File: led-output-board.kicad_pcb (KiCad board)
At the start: 2 copper layers, 80.9 x 96.4 mm, 29 parts, among them J1 DBT50G-9.5-2P, J10 DB301V-3.5-3P-GN, J2 Conn_02x08_Odd_Even, J3 DB301V-3.5-3P-GN, J4 DB301V-3.5-3P-GN, J5 DB301V-3.5-3P-GN, J6 DB301V-3.5-3P-GN, J7 DB301V-3.5-3P-GN, J8 DB301V-3.5-3P-GN, J9 DB301V-3.5-3P-GN, U1 SN74LVC8T245PWR

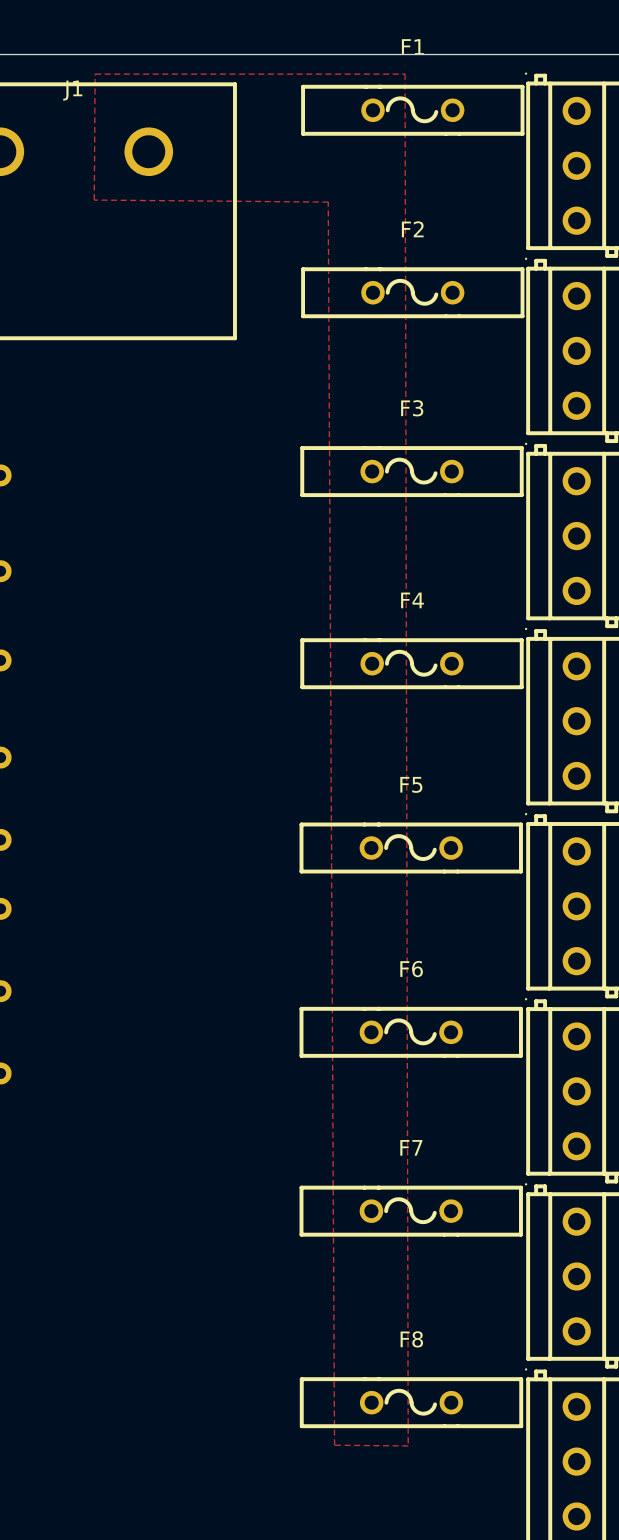
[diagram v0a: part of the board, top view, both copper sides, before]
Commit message: Widened and filled zone
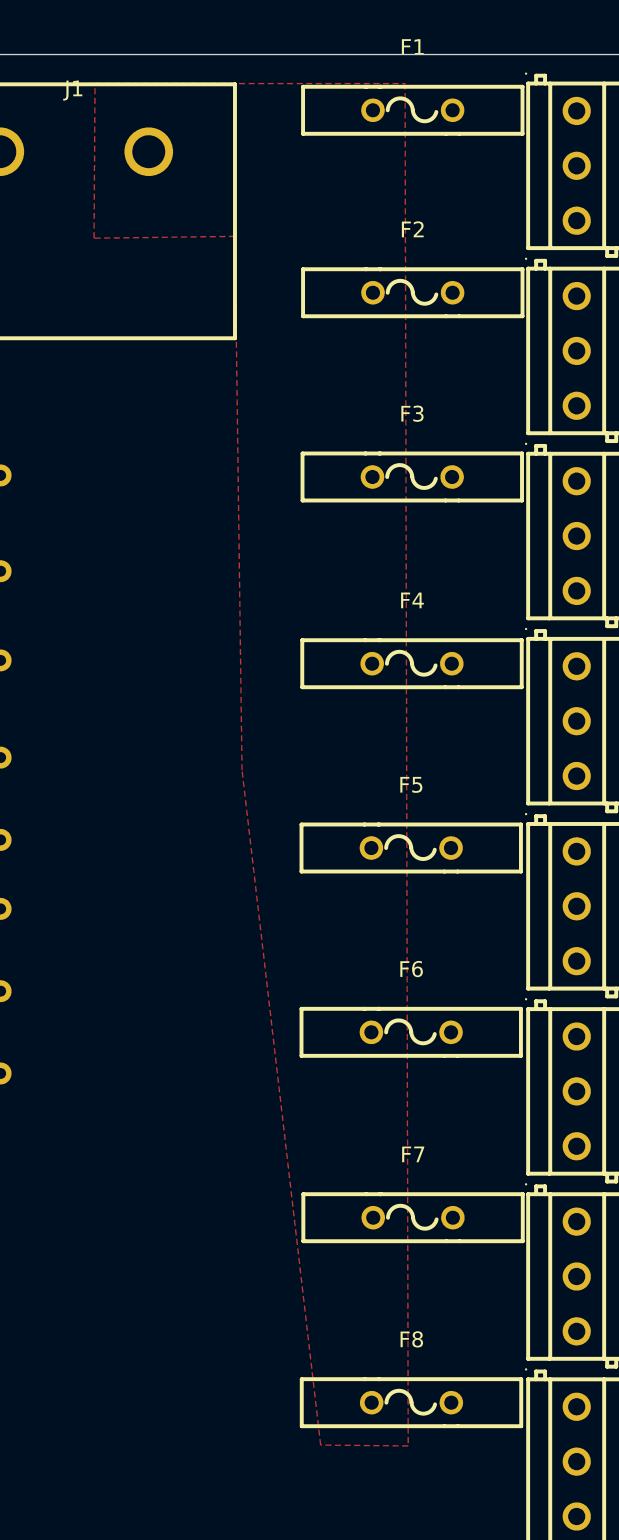
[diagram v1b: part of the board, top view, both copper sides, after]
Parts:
- moved F7 0.43 mm to (127.3, 139.4)
- moved F3 0.35 mm to (127.2, 92.2)
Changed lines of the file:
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@@
 	(footprint "easyeda2kicad:FUSE-TH_L14.0-W3.0-P5.08-D0.6"
 		(layer "F.Cu")
-		(at 127.1925 91.803929)
+		(at 127.21 92.15)
 		(property "Reference" "F3"
 			(at 0 -4 0)
@@
 	(footprint "easyeda2kicad:FUSE-TH_L14.0-W3.0-P5.08-D0.6"
 		(layer "F.Cu")
-		(at 127.1425 138.9825)
+		(at 127.26 139.4)
 		(property "Reference" "F7"
 			(at 0 -4 0)
@@
 		)
 		(min_thickness 0.25)
-		(fill
+		(fill yes
 			(thermal_gap 0.5)
 			(thermal_bridge_width 0.5)
@@
 		(polygon
 			(pts
-				(xy 106.974844 66.45) (xy 126.75 66.45) (xy 126.950022 153.959616) (xy 122.250073 153.914424) (xy 121.850065 74.612767)
-				(xy 106.924933 74.485744)
+				(xy 106.971117 67.05) (xy 126.751371 67.05) (xy 126.950022 153.959616) (xy 121.366483 153.905928)
+				(xy 116.35 110.85) (xy 115.9 76.8) (xy 106.909825 76.918169)
 			)
 		)
